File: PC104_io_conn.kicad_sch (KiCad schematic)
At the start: 14 parts, among them J13 ESQ-126-39-G-D_SAI, J15 ESQ-126-39-G-D_SAI

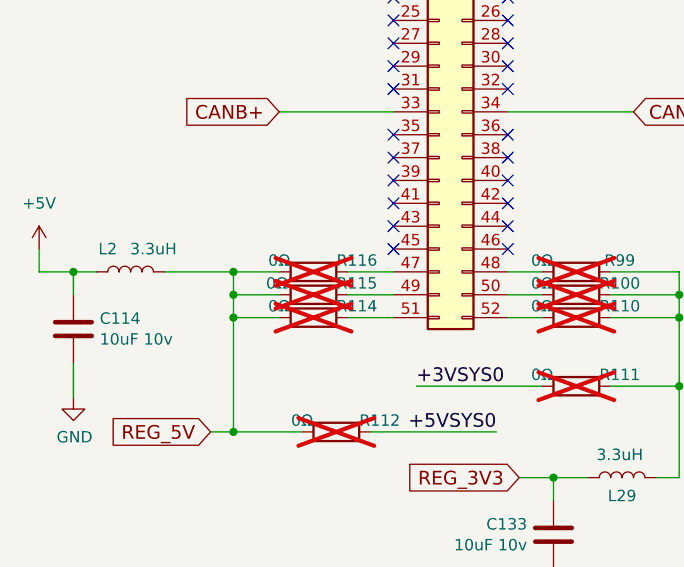
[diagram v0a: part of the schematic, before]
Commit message: Minor fixes for BOM values
Signed-off-by: Corey Minyard <corey@minyard.net>
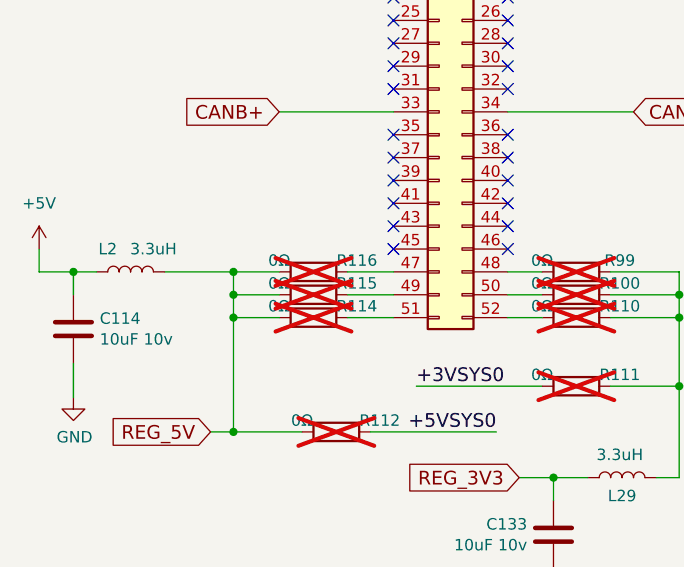
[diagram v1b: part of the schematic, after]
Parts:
- R115: value 0Ω' -> 0Ω
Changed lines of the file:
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@@
 			)
 		)
-		(property "Value" "0Ω'"
+		(property "Value" "0Ω"
 			(at 125.73 156.21 90)
 			(effects
